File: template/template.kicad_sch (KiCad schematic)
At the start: 3 parts, among them J1 B2B STLink connector, U1 STM32G474RBT6

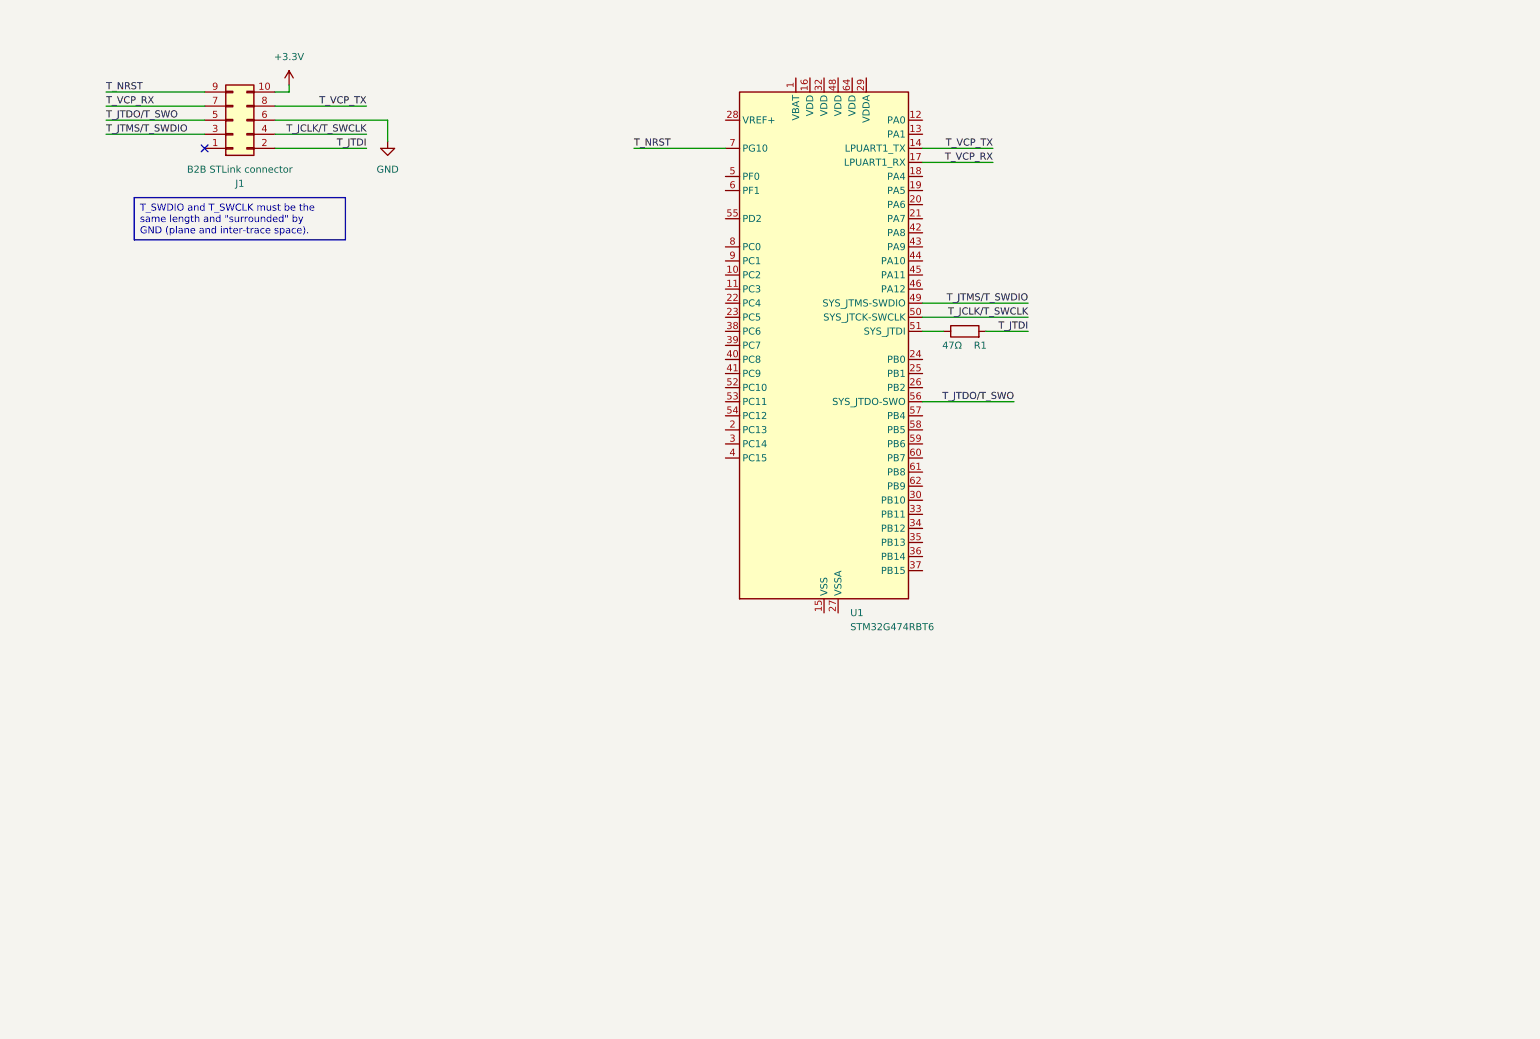
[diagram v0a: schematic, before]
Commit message: Schematics for the first version of the STM32 template
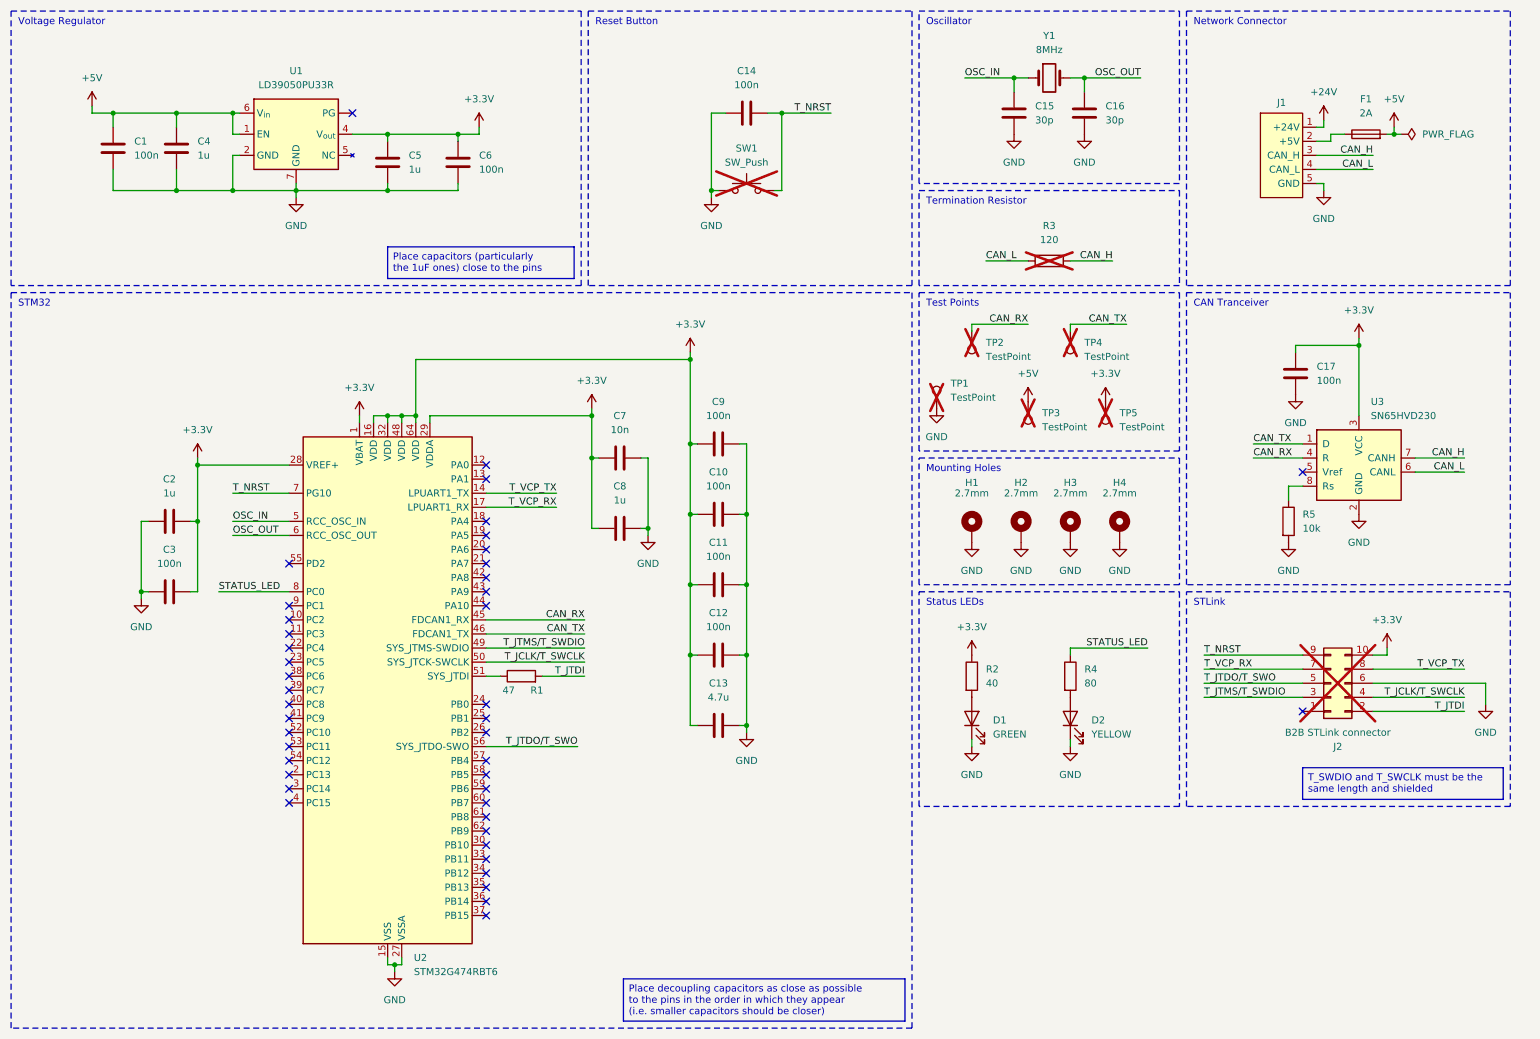
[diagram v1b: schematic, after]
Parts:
- added C1, C10, C11, C12, C14, C17, C3, C6, C9: 100n, symbol Device:C
- added C13: 4.7u, symbol Device:C
- added C15, C16: 30p, symbol Device:C
- added C2, C4, C5, C8: 1u, symbol Device:C
- added C7: 10n, symbol Device:C
- added D1: GREEN, symbol Device:LED
- added D2: YELLOW, symbol Device:LED
- added F1: 2A, symbol Device:Fuse
- added H1, H2, H3, H4: 2.7mm, MountingHole:MountingHole_2.7mm_Pad, symbol Mechanical:MountingHole_Pad
- added J1: Network Connector, symbol Exocet:Network_Connector
- added R2: 40, symbol Device:R
- added R3: 120, Resistor_THT:R_Axial_DIN0309_L9.0mm_D3.2mm_P12.70mm_Horizontal, symbol Device:R
- added R4: 80, symbol Device:R
- added R5: 10k, symbol Device:R
- added SW1: SW_Push, Button_Switch_THT:SW_PUSH_6mm, symbol Switch:SW_Push
- added TP1, TP2, TP3, TP4, TP5: TestPoint, TestPoint:TestPoint_Keystone_5005-5009_Compact, symbol Connector:TestPoint
- added U1: LD39050PU33R, Package_DFN_QFN:DFN-6-1EP_3x3mm_P0.95mm_EP1.7x2.6mm, symbol Exocet:LD39050PU33R
- added U3: SN65HVD230, Package_SO:SOIC-8_3.9x4.9mm_P1.27mm, symbol Interface_CAN_LIN:SN65HVD230
- added Y1: 8MHz, symbol Exocet:HSE_Oscillator
- J2: renamed from J1; footprint Exocet_Footprint:AVX 00-9159-010-BTB Connector -> Exocet:AVX 00-9159-010-BTB Connector; now not fitted
- R1: value 47Ω -> 47
- renumbered U1 to U2
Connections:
- net +3.3V: now also U2.1 (VBAT), U2.16 (VDD), U2.28 (VREF+), U2.29 (VDDA), U2.32 (VDD), U2.48 (VDD), U2.64 (VDD), C10.1, C11.1, C12.1, C13.1, C17.1, C2.2, C3.2, C5.1, C6.1, C7.1, C8.1, C9.1, R2.1, TP5.1, U1.4 (V_{out}), U3.3 (VCC)
- net GND: now also U2.15 (VSS), U2.27 (VSSA), U2.31 (VSS), U2.47 (VSS), U2.63 (VSS), C1.2, C10.2, C11.2, C12.2, C13.2, C14.1, C15.2, C16.2, C17.2, C2.1, C3.1, C4.2, C5.2, C6.2, C7.2, C8.2, C9.2, D1.1 (K), D2.1 (K), H1.1, H2.1, H3.1, H4.1, J1.5 (GND), R5.2, SW1.1, TP1.1, U1.2 (GND), U1.7 (GND), U3.2 (GND)
- net T_NRST: now also C14.2, SW1.2
- net CAN_RX: now reaches U2.45 (PA11)
- net CAN_RX: now also TP2.1, U3.4 (R)
- net CAN_TX: now reaches U2.46 (PA12)
- net CAN_TX: now also TP4.1, U3.1 (D)
- net OSC_IN: now reaches U2.5 (PF0)
- net OSC_IN: now also C15.1, Y1.1
- net OSC_OUT: now reaches U2.6 (PF1)
- net OSC_OUT: now also C16.1, Y1.2
- net STATUS_LED: now reaches U2.8 (PC0)
- net STATUS_LED: now also R4.1
- new net: F1.1, J1.2 (+5V)
- new net: D1.2 (A), R2.2
- new net: R5.1, U3.8 (Rs)
- new net: D2.2 (A), R4.2
- new net +24V: J1.1 (+24V)
- new net +5V: C1.1, C4.1, F1.2, TP3.1, U1.1 (EN), U1.6 (V_{in})
- new net CAN_H: J1.3 (CAN_H), R3.2, U3.7 (CANH)
- new net CAN_L: J1.4 (CAN_L), R3.1, U3.6 (CANL)
- no-connect marks 1 -> 43
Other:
- note added: "CAN Tranceiver"
- note added: "Mounting Holes"
- note added: "Network Connector"
- note added: "Oscillator"
- note added: "Reset Button"
- note added: "STLink"
- note added: "STM32"
- note added: "Status LEDs"
- note added: "Termination Resistor"
- note added: "Test Points"
- note added: "Voltage Regulator"
- moved on the sheet: R1, U2

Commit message: Add oscillator symbol
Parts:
- Y1: footprint (none) -> Exocet:Crystal_SMD_HC49-SD
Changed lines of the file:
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@@
 			)
 		)
-		(property "Footprint" ""
+		(property "Footprint" "Exocet:Crystal_SMD_HC49-SD"
 			(at 200.66 25.4 0)
 			(effects
